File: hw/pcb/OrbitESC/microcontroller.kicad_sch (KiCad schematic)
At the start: 29 parts, among them J6 CAN1, SW1 Reset, SW2 Boot, U1 TLE9250X, U11 STM32L432KBUx, U2 AT25SF081-SSHD-X, U3 24LC128

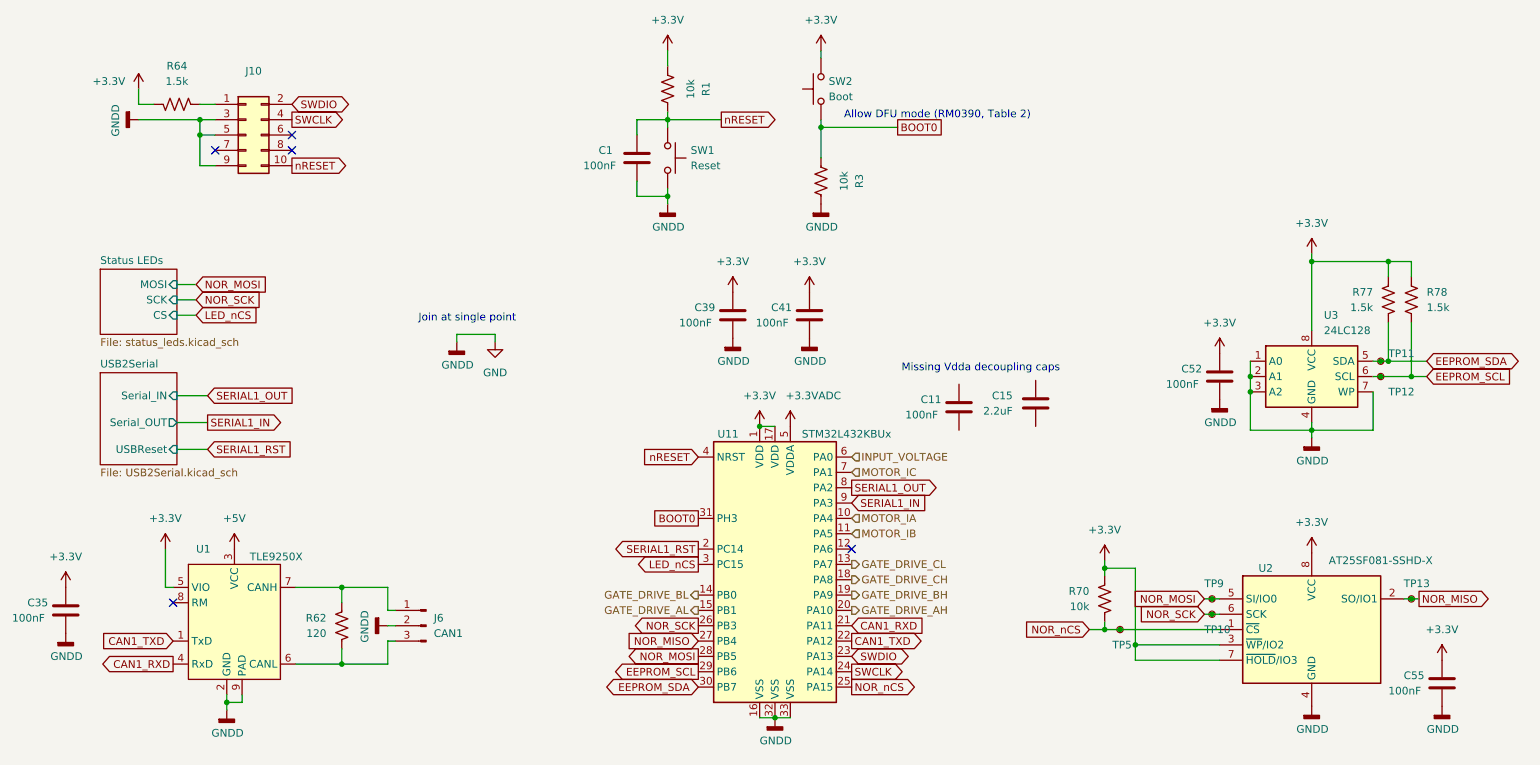
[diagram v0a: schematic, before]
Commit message: Sync lunch schematic update
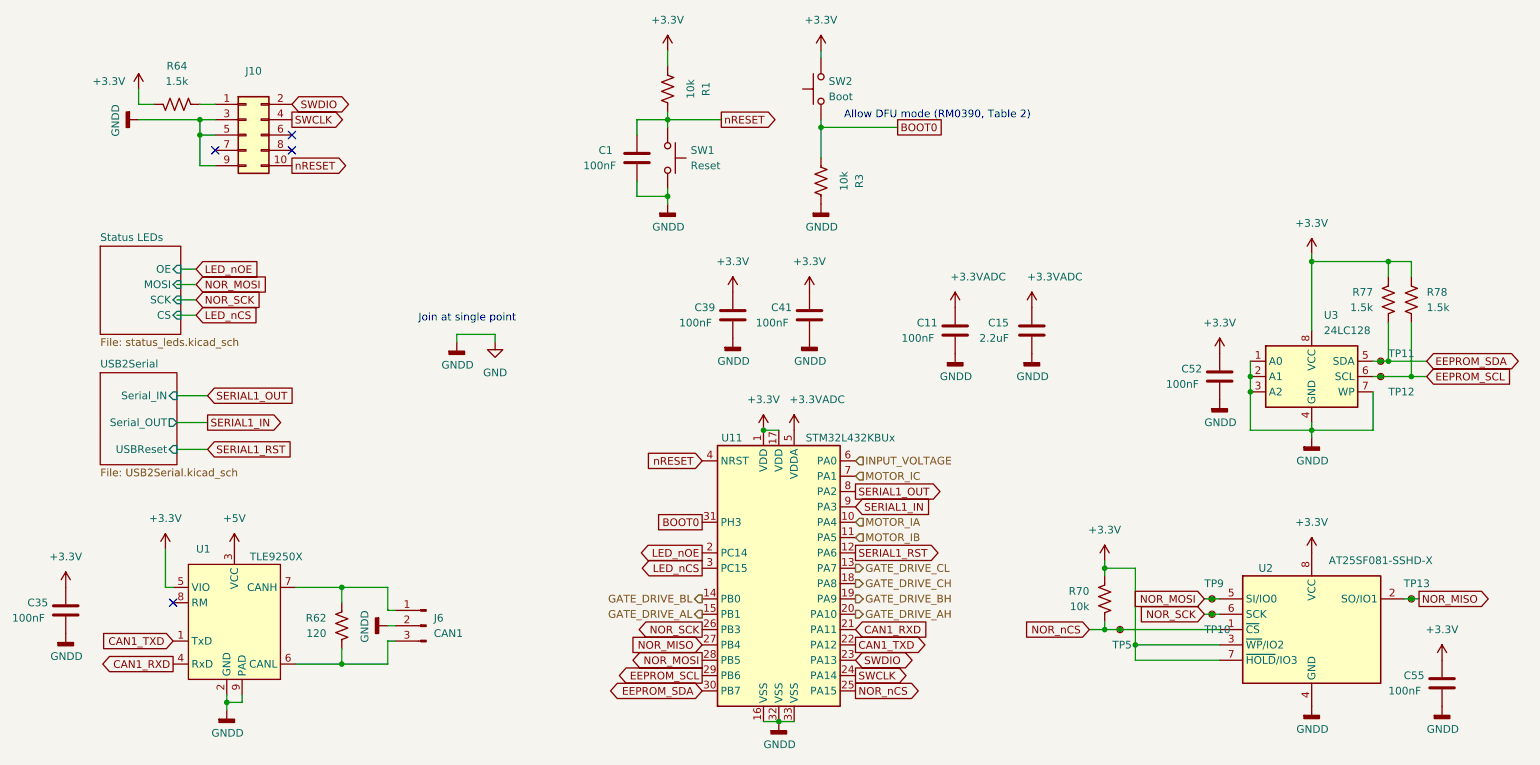
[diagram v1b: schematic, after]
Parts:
- U11: JLCPCB (none) -> C1337280
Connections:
- net +3.3VADC: now also C11.2, C15.2
- net GND: now also C11.1, C15.1
- net SERIAL1_RST: now also U11.12 (PA6); no longer U11.2 (PC14)
- new net LED_nOE: U11.2 (PC14)
- no-connect marks 5 -> 4
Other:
- sheet Status LEDs ports: added OE; removed none
- note removed: "Missing Vdda decoupling caps"
- moved on the sheet: C11, C15, U11
